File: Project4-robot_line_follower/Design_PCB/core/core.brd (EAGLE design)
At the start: 101.3 x 53.3 mm, 23 parts, among them IC1 MCP3008-I_P, IC2 AT24CP, IC4 7402N, M1 ARDUINO-NANO-3.0

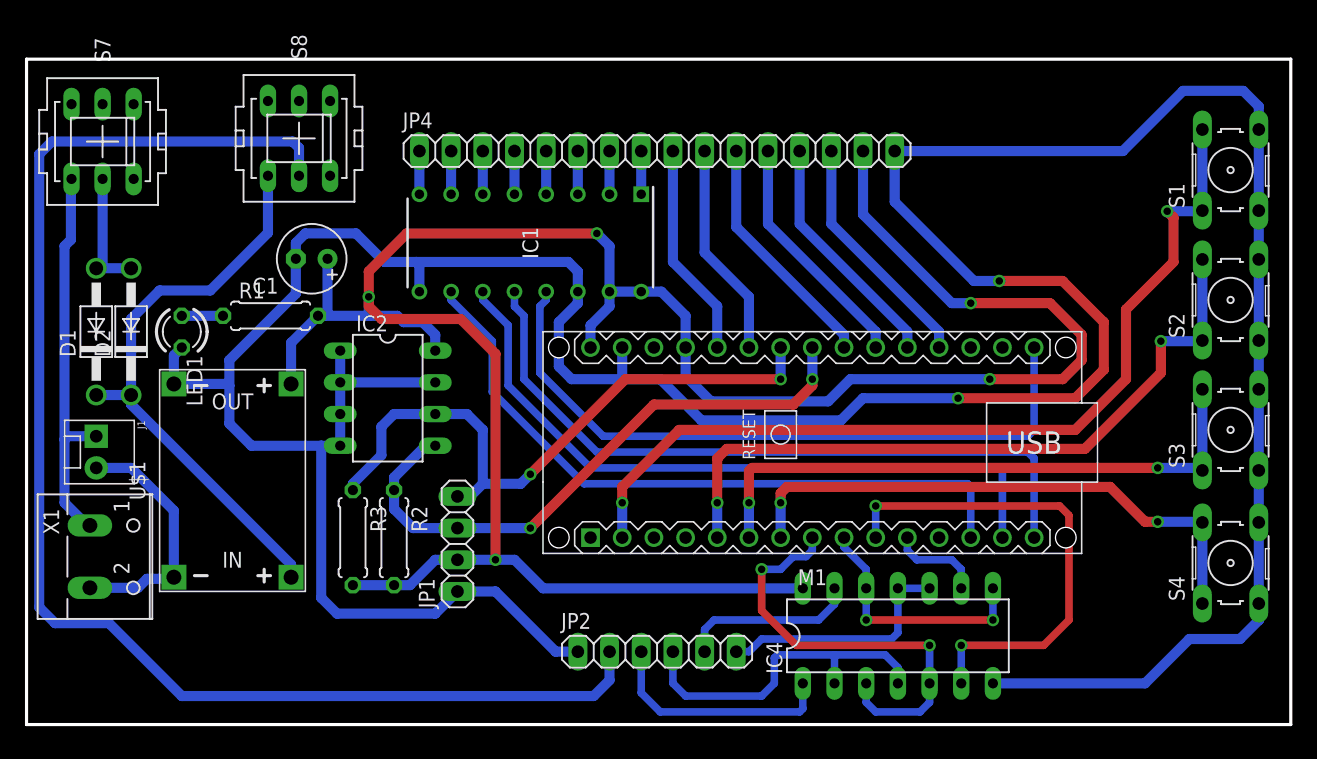
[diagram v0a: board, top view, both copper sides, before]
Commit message: rename file
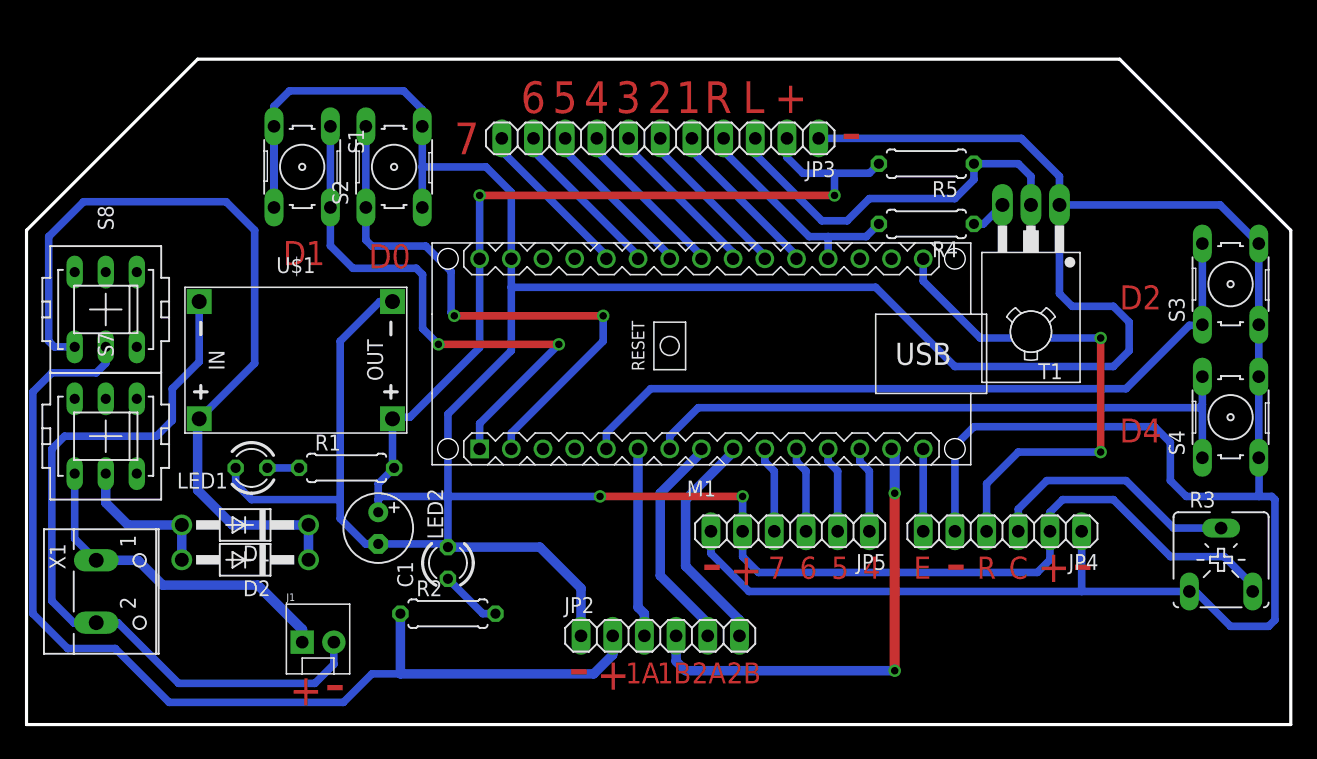
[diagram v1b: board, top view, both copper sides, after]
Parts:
- removed IC1: MCP3008-I_P, MCP3008-I_P:DIP781W56P254L1918H533Q16N
- removed IC2: AT24CP, atmel:DIL08
- removed IC4: 7402N, 74xx-us:DIL14
- removed JP1: (no value), pinhead:1X04
- added JP3: (no value), pinhead:1X11
- added JP5: (no value), pinhead:1X06
- added LED2: (no value), led:LED3MM
- added R4, R5: 1K, rcl:0207/7
- added T1: BD139, transistor-neu-to92:TO126
- JP4: device pinhead:1X16 -> pinhead:1X06
- R2: value 4.7K -> 22K
- R3: value 4.7K -> (none); device rcl:0207/7 -> pot:CA6V
- U$1: value DC-DC-STEP-DOWN-MP2307 -> (none)
- moved S1 74.4 mm to (-86.9, 54.6), turned to 270 degrees
- moved R3 69.6 mm to (-13.2, 23.1), turned to 0 degrees
- moved S2 67.9 mm to (-79.5, 54.6)
- moved JP4 41.2 mm to (-30.7, 25.4), turned to 180 degrees
- moved S7 23.6 mm to (-102.6, 33.0)
- moved J1 23.3 mm to (-86.9, 16.5), turned to 0 degrees
- moved C1 22.2 mm to (-80.8, 25.7), turned to 270 degrees
- moved S8 20.7 mm to (-102.6, 43.2)
- moved D2 20.4 mm to (-91.4, 23.1), turned to 180 degrees
- moved D1 19.6 mm to (-91.4, 25.9), turned to 180 degrees
- moved R1 13.6 mm to (-83.3, 30.5)
- moved LED1 12.3 mm to (-90.9, 30.5), turned to 180 degrees
- moved S3 11.7 mm to (-12.4, 45.2)
- moved S4 11.7 mm to (-12.4, 34.5)
- moved M1 11.4 mm to (-54.9, 39.6)
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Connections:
- removed net 1A: IC4.1, JP2.3
- removed net 1B: IC4.2, IC4.4, JP2.4
- removed net 2A: IC4.13, JP2.5
- removed net 2B: IC4.10, IC4.11, JP2.6
- removed net 5V: C1.+, IC1.15, IC1.16, IC2.8, IC4.14, JP1.2, JP4.15, M1.J2.1, M1.J2.4, R1.2, R2.2, R3.2, U$1.OUT+
- removed net A0: JP4.14, M1.J2.12
- removed net A10: IC1.5, JP4.4
- removed net A11: IC1.6, JP4.3
- removed net A12: IC1.7, JP4.2
- removed net A13: IC1.8, JP4.1
- removed net A8: IC1.3, JP4.6
- removed net A9: IC1.4, JP4.5
- removed net B5: M1.J1.7, S4.1, S4.2
- removed net B6: M1.J1.12
- removed net CS: IC1.10, M1.J1.13
- removed net DIR1: IC4.6, M1.J1.10
- removed net DIR2: IC4.9, M1.J1.11
- removed net MISO: IC1.12, M1.J1.15
- removed net MOSI: IC1.11, M1.J1.14
- removed net N$4: JP2.2, S8.2
- removed net PWM1: IC4.3, IC4.5, M1.J1.8
- removed net PWM2: IC4.12, IC4.8, M1.J1.9
- removed net SCK: IC1.13, M1.J2.15
- removed net SCL: IC2.6, JP1.4, M1.J2.7, R3.1
- removed net SDA: IC2.5, JP1.3, M1.J2.8, R2.1
- new net 12VM: JP2.2, R2.1, S8.2
- new net 5VIN: C1.+, JP3.2, JP4.2, JP5.5, M1.J2.1, R1.2, R3.E, R5.2, U$1.OUT+
- new net D4: JP5.1, M1.J1.13
- new net D5: JP5.2, M1.J1.12
- new net D6: JP5.3, M1.J1.11
- new net D7: JP5.4, M1.J1.10
- new net E: JP4.6, M1.J1.15
- new net L: JP3.3, R5.1, T1.2
- new net N$6: LED2.A, R2.2
- new net N$7: R4.1, T1.3
- new net N$8: JP4.3, R3.S
- new net N$9: M1.J2.4
- new net PWM1A: JP2.6, M1.J1.9
- new net PWM1B: JP2.5, M1.J1.8
- new net PWM2A: JP2.4, M1.J1.14
- new net PWM2B: JP2.3, M1.J1.6
- new net R: JP3.4, M1.J2.12, R4.2
- new net RS: JP4.4, M1.J2.15
- net A1: now also JP3.5; no longer JP4.13
- net A2: now also JP3.6; no longer JP4.12
- net A3: now also JP3.7; no longer JP4.11
- net A4: now also JP3.8, M1.J2.8; no longer JP4.10, M1.J2.6
- net A5: now also JP3.9, M1.J2.7; no longer JP4.9, M1.J2.5
- net A6: now also JP3.10, M1.J2.6; no longer IC1.1, JP4.8
- net A7: now also JP3.11, M1.J2.5; no longer IC1.2, JP4.7
- net B1: now also S1.1, S1.2
- net B2: now also S2.1, S2.2; no longer S1.1, S1.2
- net B3: now also S3.1, S3.2; no longer S2.1, S2.2
- net B4: now also M1.J1.7, S4.1, S4.2; no longer M1.J1.6, S3.1, S3.2
- net GND: now also JP3.1, JP4.1, JP4.5, JP5.6, LED2.K, R3.A, T1.1; no longer IC1.14, IC1.9, IC2.1, IC2.2, IC2.3, IC2.4, IC2.7, IC4.7, JP1.1, JP4.16
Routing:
- net N$5: track 309.4 -> 0.00 mm
- net N$3: track 309.4 -> 0.00 mm
- net 5V: track 196.8 -> 0.00 mm, vias 5 -> 0
- net 5VIN: track 0.00 -> 153.1 mm, vias 0 -> 4
- net N$4: track 111.5 -> 0.00 mm
- net 12VM: track 0.00 -> 83.2 mm
- net GND: track 294.8 -> 359.8 mm, vias 2 -> 0
- net MISO: track 57.2 -> 0.00 mm
- net MOSI: track 56.2 -> 0.00 mm
- net SCK: track 55.3 -> 0.00 mm
- net CS: track 55.0 -> 0.00 mm
- net SCL: track 51.8 -> 0.00 mm, vias 2 -> 0
- net SDA: track 48.8 -> 0.00 mm, vias 2 -> 0
- net B5: track 45.3 -> 0.00 mm, vias 2 -> 0
- net B1: track 0.00 -> 44.7 mm, vias 0 -> 2
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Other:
- outline, holes or cut-outs redrawn
- board text added: "+"
- board text added: "-"
- board text added: "1"
- board text added: "1A"
- board text added: "1B"
- board text added: "2"
- board text added: "2A"
- board text added: "2B"
- board text added: "3"
- board text added: "4"
- board text added: "5"
- board text added: "6"
- board text added: "7"
- board text added: "C"
- board text added: "D0"
- board text added: "D1"
- board text added: "D2"
- board text added: "D4"
- board text added: "E"
- board text added: "L"
- board text added: "R"
